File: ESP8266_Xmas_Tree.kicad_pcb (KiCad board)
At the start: 2 copper layers, 174.3 x 184.8 mm, 46 parts, among them U1 WeMos_D1_mini

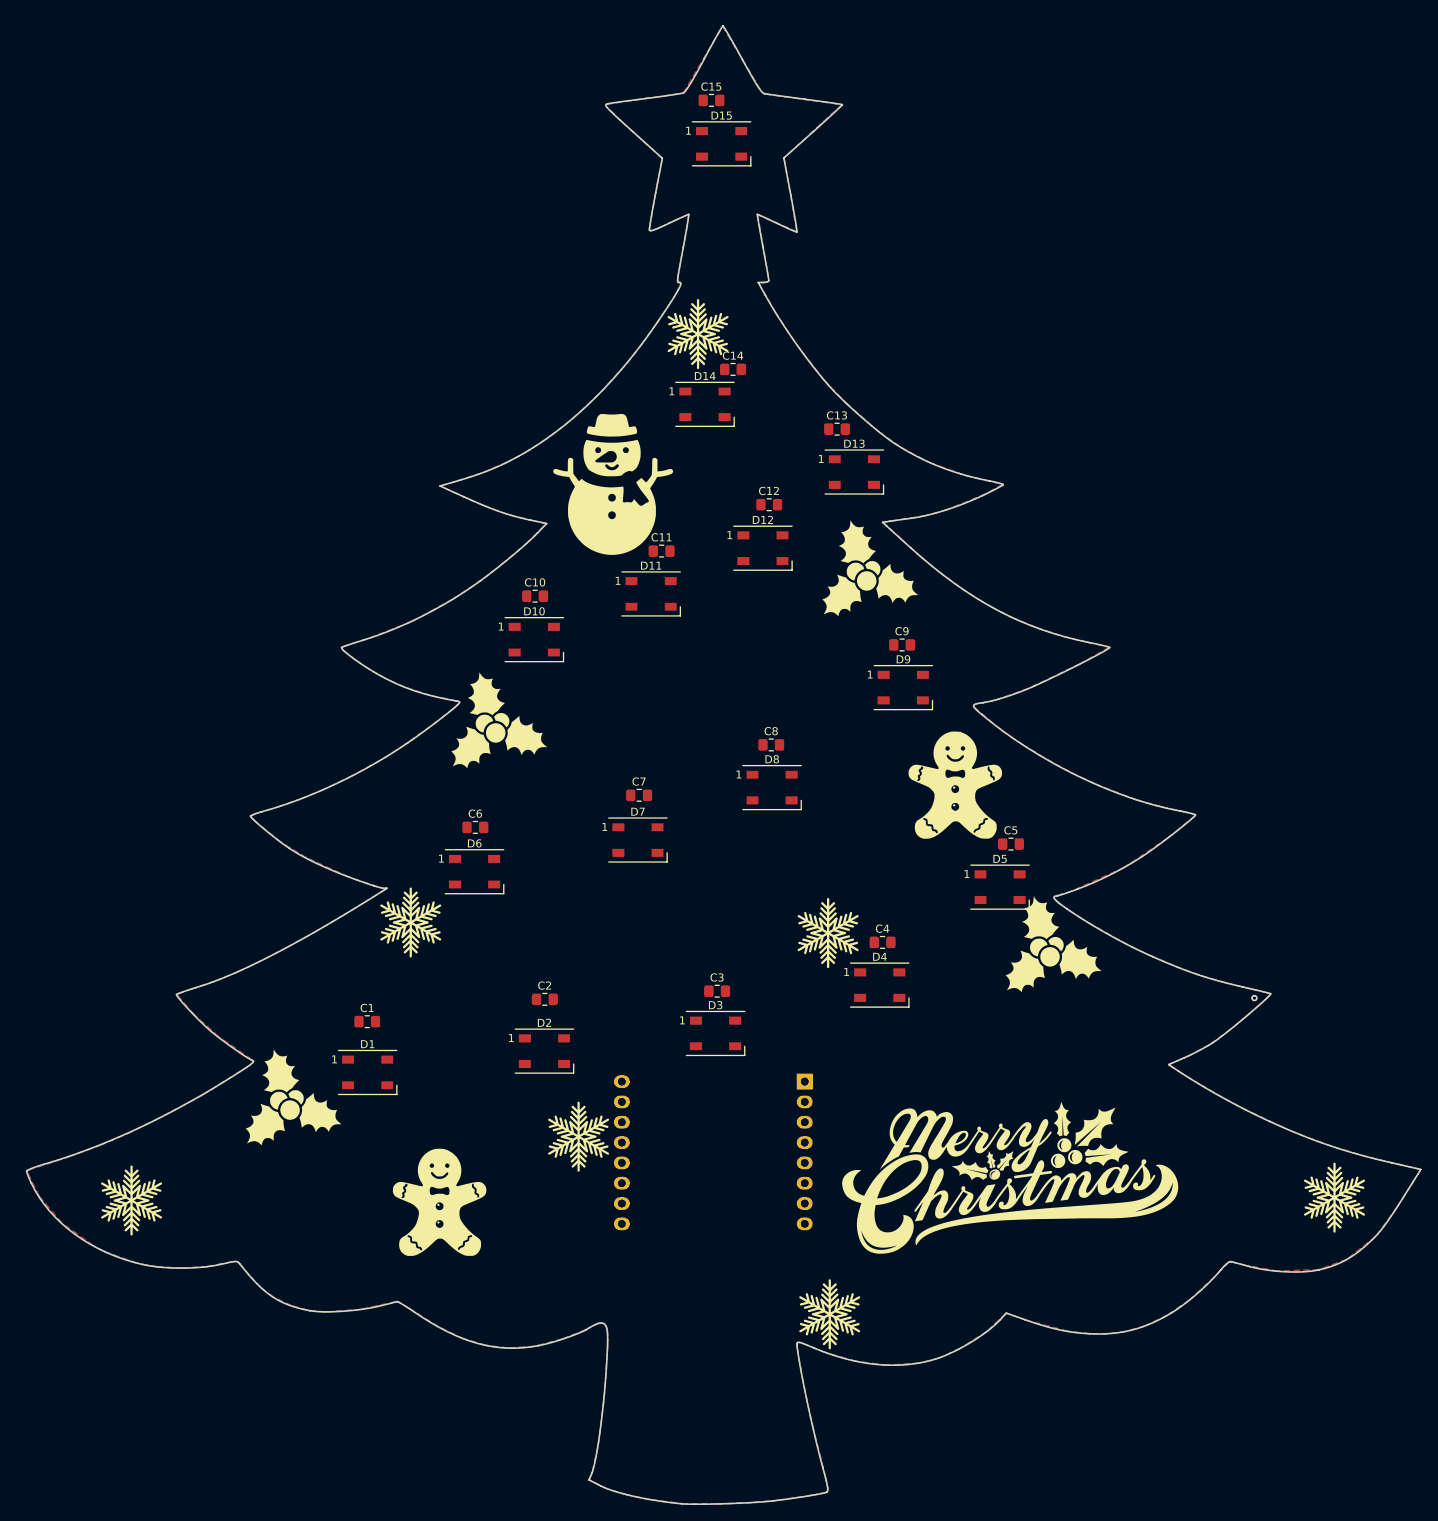
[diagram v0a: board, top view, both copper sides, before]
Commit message: adding Edge Cuts, Silkscreen an filled zones from SVG files
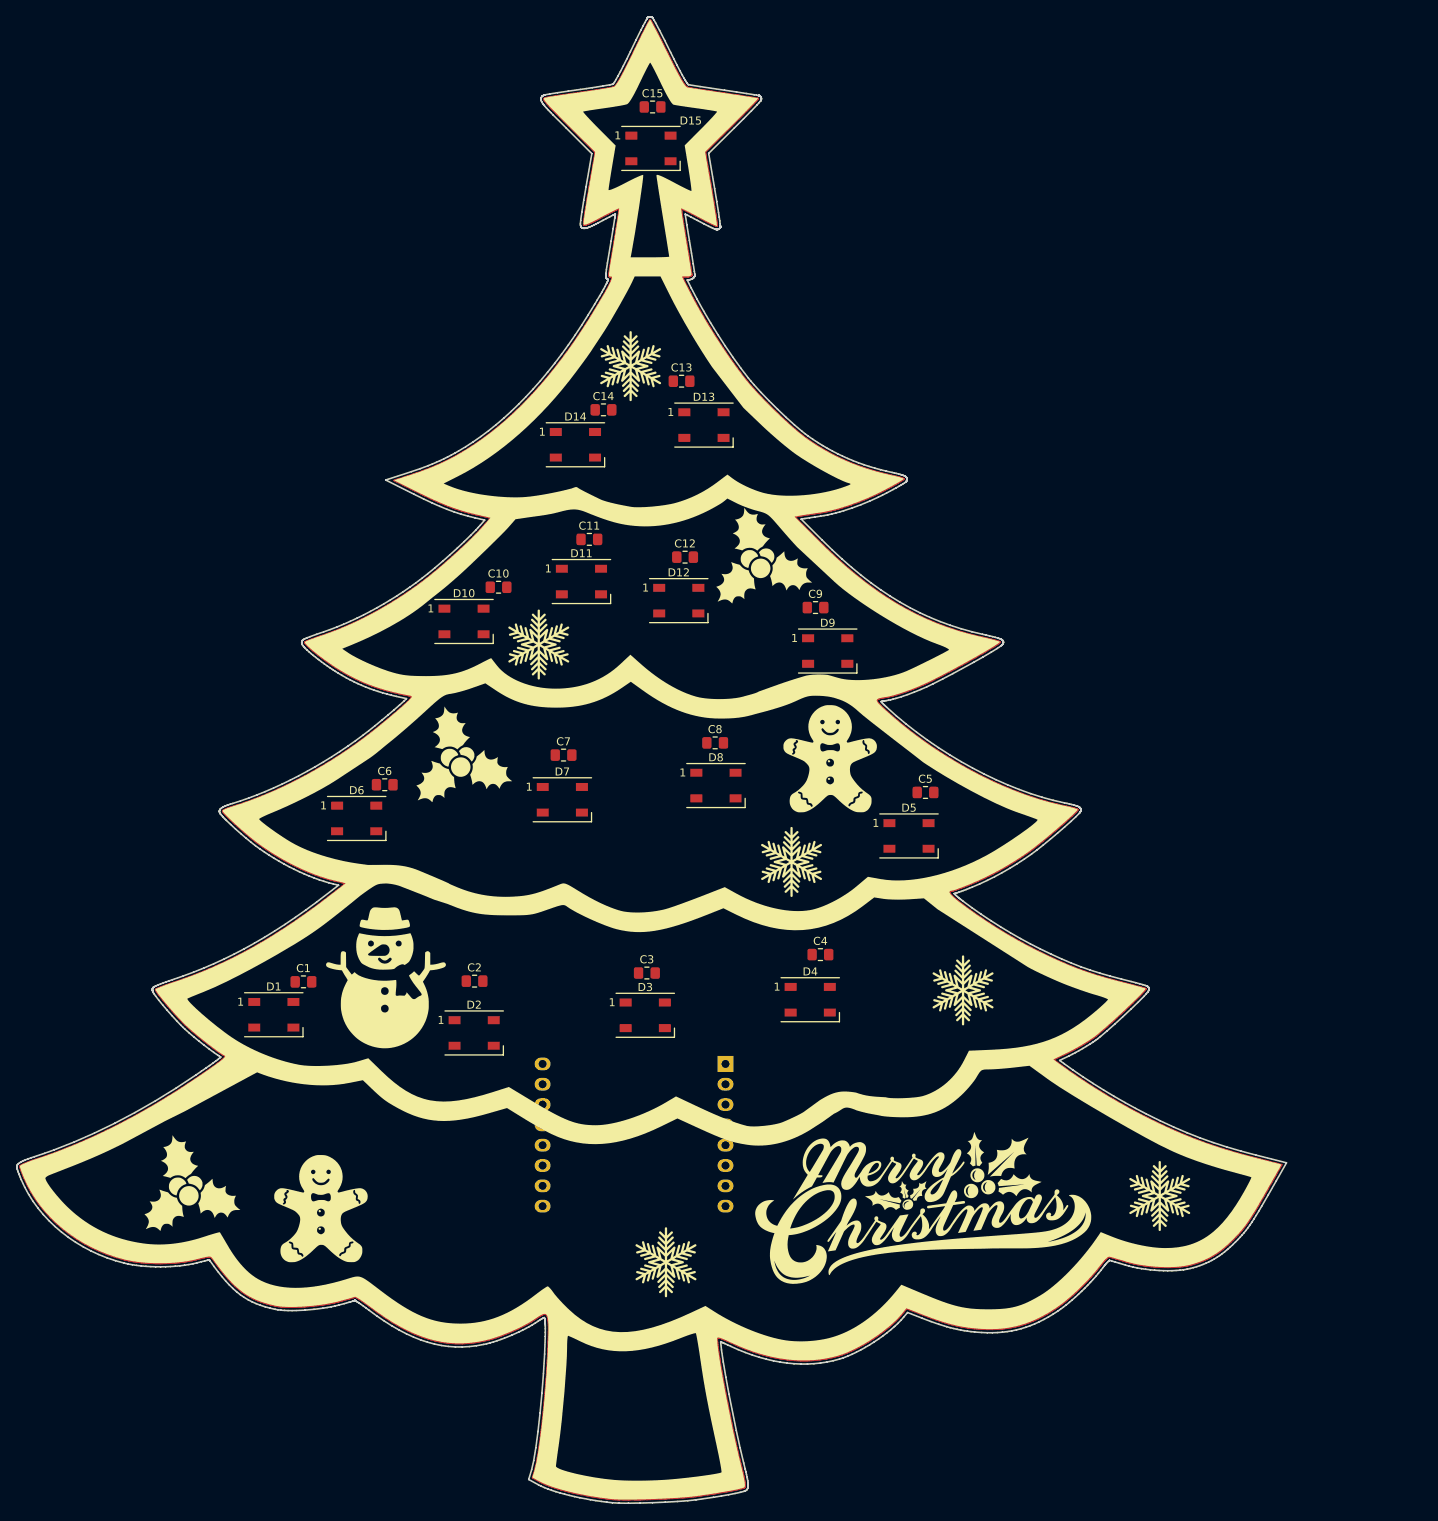
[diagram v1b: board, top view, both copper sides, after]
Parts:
- removed the G*** at (136.3, 199.6)
- removed the G*** at (251.6, 167.6)
- moved G*** 69.6 mm to (240.3, 173.4)
- moved G*** 67.9 mm to (168.1, 171.8)
- moved G*** 61.7 mm to (187.2, 130.1)
- moved G*** 21.8 mm to (264.9, 199.1)
- moved G*** 21.5 mm to (203.1, 207.4)
- moved C13 20.3 mm to (205.1, 97.2)
- moved D13 19.7 mm to (207.9, 102.7)
- moved C14 17.0 mm to (195.3, 100.8)
- moved D14 17.0 mm to (191.8, 105.2)
- moved G*** 16.6 mm to (144.0, 197.5)
- moved D6 16.2 mm to (164.5, 151.9)
- moved G*** 16.0 mm to (223.7, 144.3)
- moved G*** 14.9 mm to (160.0, 200.5)
- moved D1 13.8 mm to (154.1, 176.4)
- moved G*** 13.4 mm to (215.4, 119.0)
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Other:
- board size 174.3 x 184.8 mm -> 158.7 x 185.8 mm
